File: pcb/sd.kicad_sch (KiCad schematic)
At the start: 8 parts, among them J1 Micro_SD_Card_Det2, J2 Conn_01x09

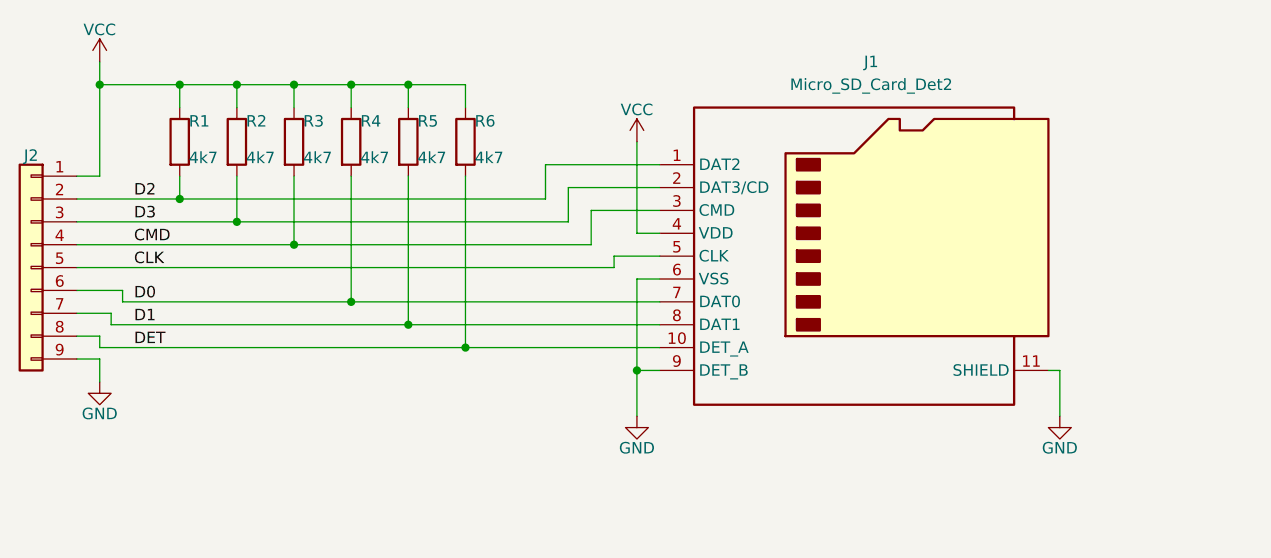
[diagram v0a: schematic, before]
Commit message: Ready for order
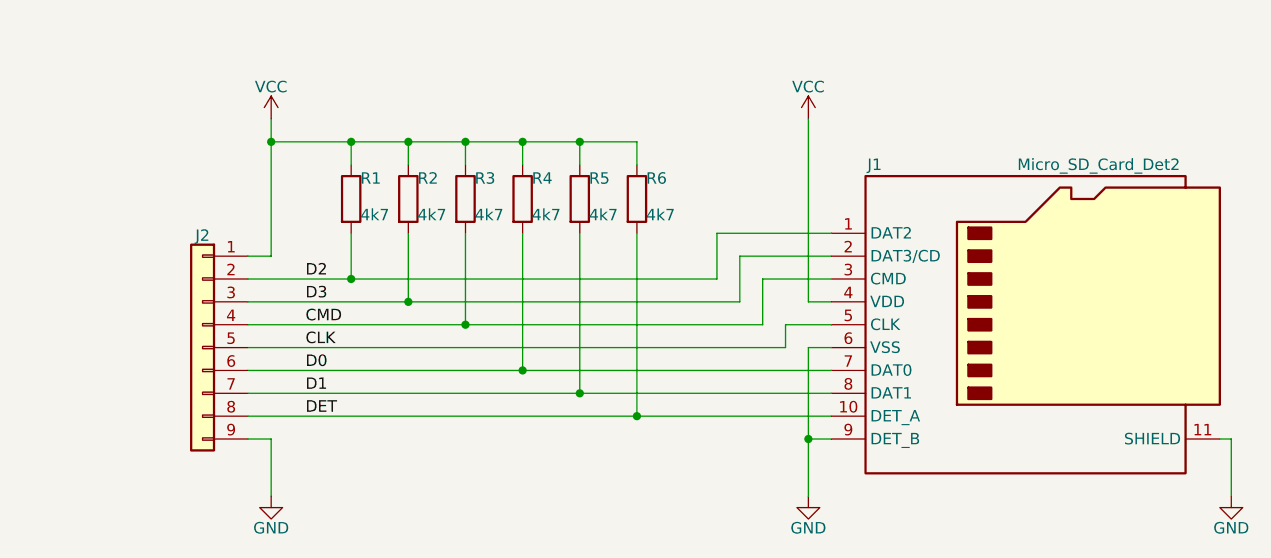
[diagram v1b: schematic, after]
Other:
- moved on the sheet: J1, J2, R1, R2, R3, R4, R5, R6
